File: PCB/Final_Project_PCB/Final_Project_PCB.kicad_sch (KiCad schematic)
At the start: 14 parts

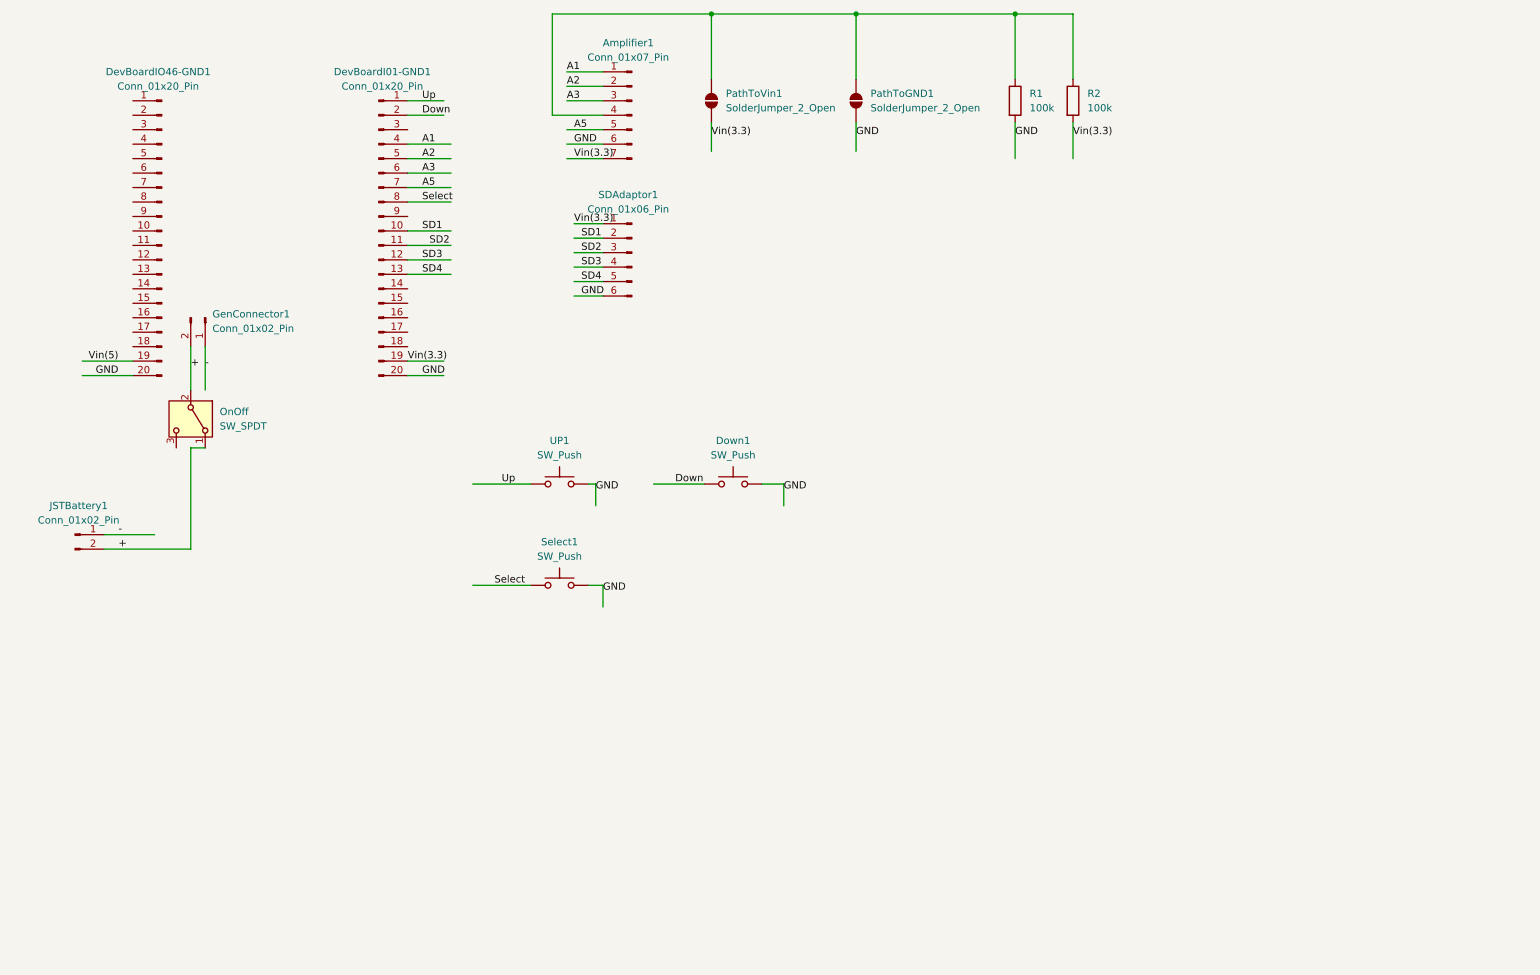
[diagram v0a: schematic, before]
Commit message: Schematic Finished
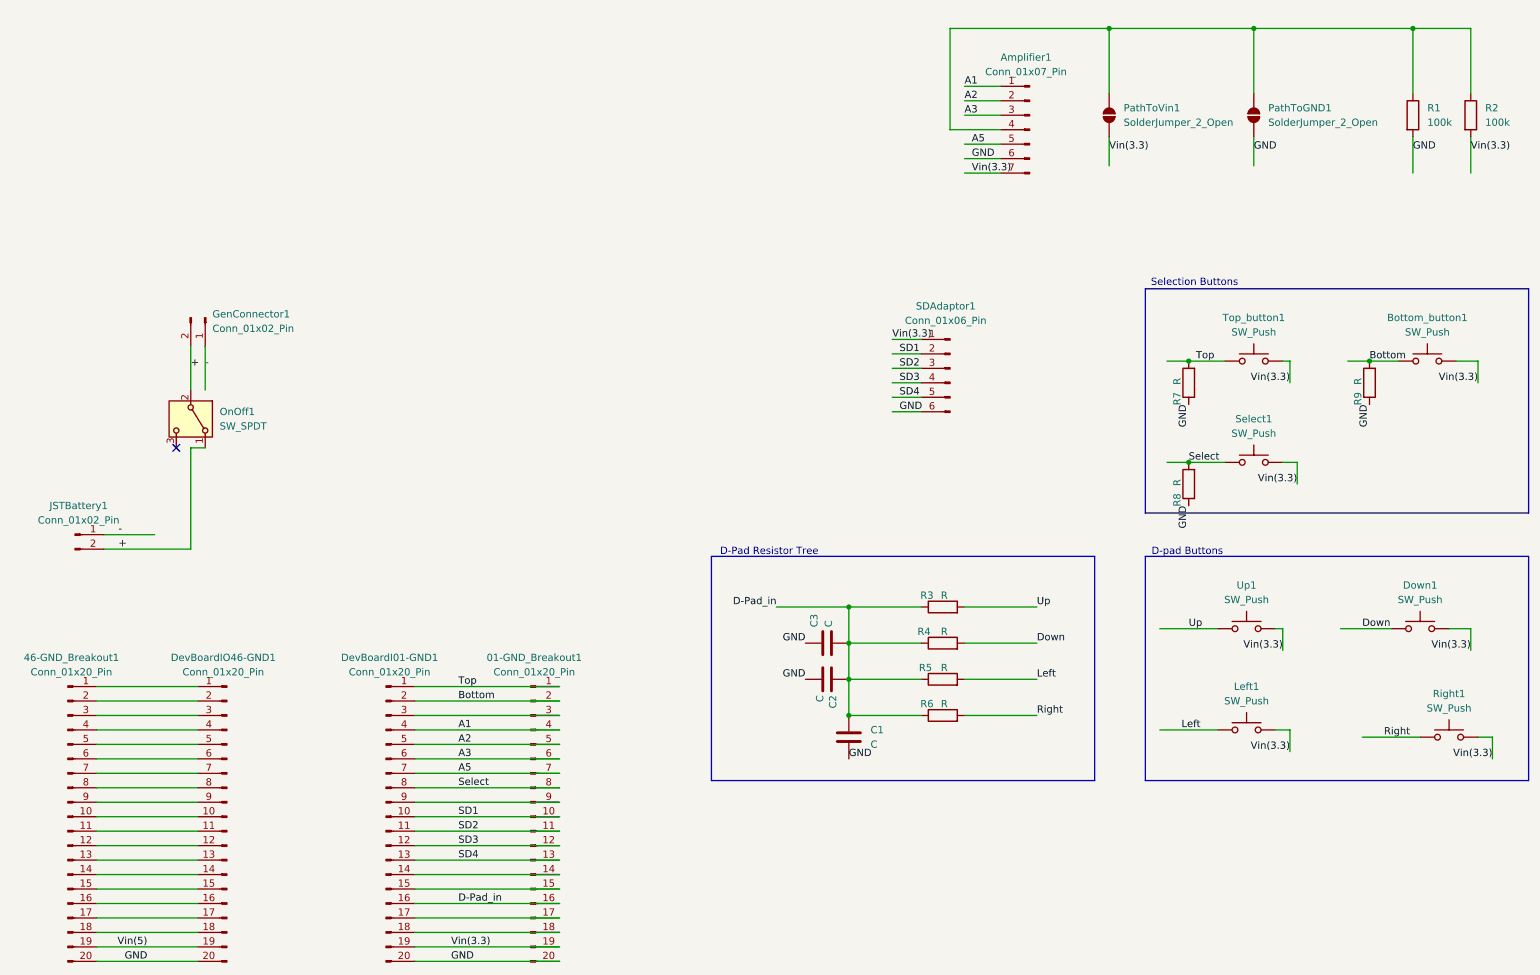
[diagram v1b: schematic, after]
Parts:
- added 01-GND_Breakout1, 46-GND_Breakout1: Conn_01x20_Pin, Connector_PinHeader_2.54mm:PinHeader_1x20_P2.54mm_Vertical, symbol Connector:Conn_01x20_Pin
- added C1, C2, C3: C, Capacitor_SMD:C_0805_2012Metric, symbol Device:C
- added Down1, Left1, Right1, Up1: SW_Push, Button_Switch_SMD:SW_SPST_PTS810, symbol Switch:SW_Push
- added R3, R4, R5, R6, R7, R8, R9: R, Resistor_SMD:R_0201_0603Metric, symbol Device:R
- renumbered Down1 to Bottom_button1, OnOff to OnOff1, UP1 to Top_button1
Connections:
- net A1: now also 01-GND_Breakout1.4 (Pin_4)
- net A2: now also 01-GND_Breakout1.5 (Pin_5)
- net A3: now also 01-GND_Breakout1.6 (Pin_6)
- net A5: now also 01-GND_Breakout1.7 (Pin_7)
- net Down: now also Down1.1, R4.2; no longer Bottom_button1.1, DevBoardI01-GND1.2 (Pin_2)
- net GND: now also 01-GND_Breakout1.20 (Pin_20), 46-GND_Breakout1.20 (Pin_20), C1.1, C2.1, C3.2, R7.1, R8.1, R9.1; no longer Bottom_button1.2, Select1.2, Top_button1.2
- net SD1: now also 01-GND_Breakout1.10 (Pin_10)
- net SD2: now also 01-GND_Breakout1.11 (Pin_11)
- net SD3: now also 01-GND_Breakout1.12 (Pin_12)
- net SD4: now also 01-GND_Breakout1.13 (Pin_13)
- net Select: now also 01-GND_Breakout1.8 (Pin_8), R8.2
- net Up: now also R3.2, Up1.1; no longer DevBoardI01-GND1.1 (Pin_1), Top_button1.1
- net Vin(3.3): now also Bottom_button1.2, Select1.2, Top_button1.2, 01-GND_Breakout1.19 (Pin_19), Down1.2, Left1.2, Right1.2, Up1.2
- net Vin(5): now also 46-GND_Breakout1.19 (Pin_19)
- net at DevBoardIO46-GND1.1 (Pin_1): now also 46-GND_Breakout1.1 (Pin_1)
- net at DevBoardIO46-GND1.10 (Pin_10): now also 46-GND_Breakout1.10 (Pin_10)
- net at DevBoardIO46-GND1.11 (Pin_11): now also 46-GND_Breakout1.11 (Pin_11)
- net at DevBoardIO46-GND1.12 (Pin_12): now also 46-GND_Breakout1.12 (Pin_12)
- net at DevBoardIO46-GND1.13 (Pin_13): now also 46-GND_Breakout1.13 (Pin_13)
- net at DevBoardIO46-GND1.14 (Pin_14): now also 46-GND_Breakout1.14 (Pin_14)
- net at DevBoardIO46-GND1.15 (Pin_15): now also 46-GND_Breakout1.15 (Pin_15)
- net at DevBoardIO46-GND1.16 (Pin_16): now also 46-GND_Breakout1.16 (Pin_16)
- net at DevBoardIO46-GND1.17 (Pin_17): now also 46-GND_Breakout1.17 (Pin_17)
- net at DevBoardIO46-GND1.18 (Pin_18): now also 46-GND_Breakout1.18 (Pin_18)
- net at DevBoardIO46-GND1.2 (Pin_2): now also 46-GND_Breakout1.2 (Pin_2)
- net at DevBoardIO46-GND1.3 (Pin_3): now also 46-GND_Breakout1.3 (Pin_3)
- net at DevBoardIO46-GND1.4 (Pin_4): now also 46-GND_Breakout1.4 (Pin_4)
- net at DevBoardIO46-GND1.5 (Pin_5): now also 46-GND_Breakout1.5 (Pin_5)
- net at DevBoardIO46-GND1.6 (Pin_6): now also 46-GND_Breakout1.6 (Pin_6)
- net at DevBoardIO46-GND1.7 (Pin_7): now also 46-GND_Breakout1.7 (Pin_7)
- net at DevBoardIO46-GND1.8 (Pin_8): now also 46-GND_Breakout1.8 (Pin_8)
- net at DevBoardIO46-GND1.9 (Pin_9): now also 46-GND_Breakout1.9 (Pin_9)
- net at DevBoardI01-GND1.14 (Pin_14): now also 01-GND_Breakout1.14 (Pin_14)
- net at DevBoardI01-GND1.15 (Pin_15): now also 01-GND_Breakout1.15 (Pin_15)
- net D-Pad_in: now reaches DevBoardI01-GND1.16 (Pin_16)
- net D-Pad_in: now also 01-GND_Breakout1.16 (Pin_16), C1.2, C2.2, C3.1, R3.1, R4.1, R5.1, R6.1
- net at DevBoardI01-GND1.17 (Pin_17): now also 01-GND_Breakout1.17 (Pin_17)
- net at DevBoardI01-GND1.18 (Pin_18): now also 01-GND_Breakout1.18 (Pin_18)
- net at DevBoardI01-GND1.3 (Pin_3): now also 01-GND_Breakout1.3 (Pin_3)
- net at DevBoardI01-GND1.9 (Pin_9): now also 01-GND_Breakout1.9 (Pin_9)
- new net Bottom: 01-GND_Breakout1.2 (Pin_2), Bottom_button1.1, DevBoardI01-GND1.2 (Pin_2), R9.2
- new net Left: Left1.1, R5.2
- new net Right: R6.2, Right1.1
- new net Top: 01-GND_Breakout1.1 (Pin_1), DevBoardI01-GND1.1 (Pin_1), R7.2, Top_button1.1
- no-connect marks 0 -> 1
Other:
- note added: "D-Pad Resistor Tree"
- note added: "D-pad Buttons"
- note added: "Selection Buttons"
- moved on the sheet: Amplifier1, Bottom_button1, DevBoardI01-GND1, DevBoardIO46-GND1, PathToGND1, PathToVin1, R1, R2, SDAdaptor1, Select1, Top_button1
